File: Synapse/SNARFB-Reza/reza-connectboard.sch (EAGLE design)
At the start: 6 parts

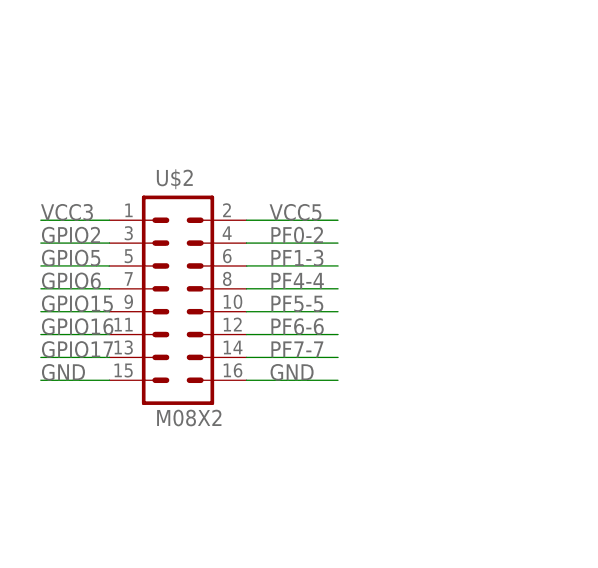
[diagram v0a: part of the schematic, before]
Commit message: comp sync
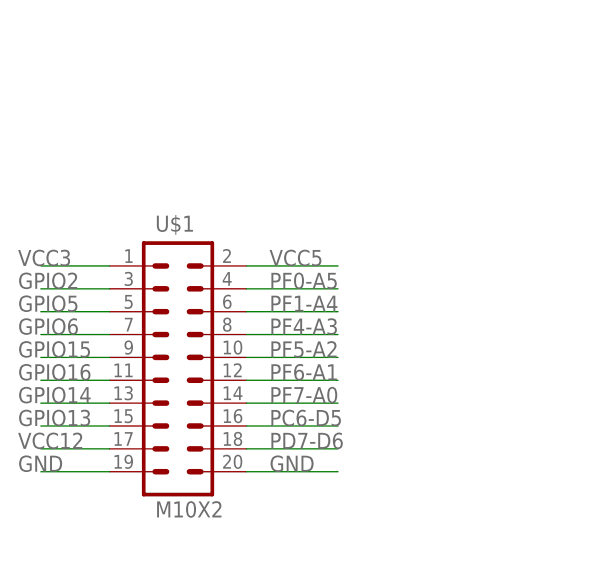
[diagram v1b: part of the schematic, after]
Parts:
- removed U$2: M08X2, SparkFun-Connectors:M08X2
- added U$1: M10X2, SparkFun-Connectors:M10X2
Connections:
- removed net GPIO17: U$2.13
- removed net PF0-2: U$2.4
- removed net PF1-3: U$2.6
- removed net PF4-4: U$2.8
- removed net PF5-5: U$2.10
- removed net PF6-6: U$2.12
- removed net PF7-7: U$2.14
- new net GPIO13: U$1.15
- new net GPIO14: U$1.13
- new net PC6-D5: U$1.16
- new net PD7-D6: U$1.18
- new net PF0-A5: U$1.4
- new net PF1-A4: U$1.6
- new net PF4-A3: U$1.8
- new net PF5-A2: U$1.10
- new net PF6-A1: U$1.12
- new net PF7-A0: U$1.14
- new net VCC12: U$1.17
- net GND: now also U$1.19, U$1.20; no longer U$2.15, U$2.16
- net GPIO15: now also U$1.9; no longer U$2.9
- net GPIO16: now also U$1.11; no longer U$2.11
- net GPIO2: now also U$1.3; no longer U$2.3
- net GPIO5: now also U$1.5; no longer U$2.5
- net GPIO6: now also U$1.7; no longer U$2.7
- net VCC3: now also U$1.1; no longer U$2.1
- net VCC5: now also U$1.2; no longer U$2.2
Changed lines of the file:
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@@
 <class number="0" name="default" width="0.254" drill="0">
+</class>
+<class number="1" name="smallsignal" width="0.1524" drill="0">
+</class>
+<class number="2" name="Power" width="0.508" drill="0">
 </class>
 </classes>
 <parts>
-<part name="U$2" library="SparkFun-Connectors" deviceset="M08X2" device=""/>
 <part name="JP1" library="SparkFun-Connectors" deviceset="M02" device="3.5MM"/>
 <part name="JP2" library="SparkFun-Connectors" deviceset="M02" device="3.5MM"/>
@@
 <part name="JP4" library="SparkFun-Connectors" deviceset="M02" device="3.5MM"/>
 <part name="JP5" library="SparkFun-Connectors" deviceset="M02" device="3.5MM"/>
+<part name="U$1" library="SparkFun-Connectors" deviceset="M10X2" device=""/>
 </parts>
 <sheets>
@@
 </plain>
 <instances>
-<instance part="U$2" gate="G$1" x="35.56" y="30.48"/>
 <instance part="JP1" gate="G$1" x="88.9" y="71.12"/>
 <instance part="JP2" gate="G$1" x="88.9" y="60.96"/>
@@
 <instance part="JP4" gate="G$1" x="88.9" y="22.86"/>
 <instance part="JP5" gate="G$1" x="88.9" y="10.16"/>
+<instance part="U$1" gate="G$1" x="35.56" y="25.4"/>
 </instances>
 <busses>
@@
 <net name="GND" class="0">
 <segment>
-<pinref part="U$2" gate="G$1" pin="15"/>
-<wire x1="27.94" y1="22.86" x2="20.32" y2="22.86" width="0.1524" layer="91"/>
-<label x="20.32" y="22.86" size="1.778" layer="95"/>
+<pinref part="U$1" gate="G$1" pin="19"/>
+<wire x1="27.94" y1="12.7" x2="20.32" y2="12.7" width="0.1524" layer="91"/>
+<label x="17.78" y="12.7" size="1.778" layer="95"/>
 </segment>
 <segment>
-<pinref part="U$2" gate="G$1" pin="16"/>
+<pinref part="U$1" gate="G$1" pin="20"/>
+<wire x1="43.18" y1="12.7" x2="53.34" y2="12.7" width="0.1524" layer="91"/>
+<label x="45.72" y="12.7" size="1.778" layer="95"/>
+</segment>
+</net>
+<net name="GPIO2" class="0">
+<segment>
+<pinref part="U$1" gate="G$1" pin="3"/>
+<wire x1="27.94" y1="33.02" x2="20.32" y2="33.02" width="0.1524" layer="91"/>
+<label x="17.78" y="33.02" size="1.778" layer="95"/>
+</segment>
+</net>
+<net name="GPIO5" class="0">
+<segment>
+<pinref part="U$1" gate="G$1" pin="5"/>
+<wire x1="27.94" y1="30.48" x2="20.32" y2="30.48" width="0.1524" layer="91"/>
+<label x="17.78" y="30.48" size="1.778" layer="95"/>
+</segment>
+</net>
+<net name="GPIO6" class="0">
+<segment>
+<pinref part="U$1" gate="G$1" pin="7"/>
+<wire x1="27.94" y1="27.94" x2="20.32" y2="27.94" width="0.1524" layer="91"/>
+<label x="17.78" y="27.94" size="1.778" layer="95"/>
+</segment>
+</net>
+<net name="GPIO16" class="0">
+<segment>
+<pinref part="U$1" gate="G$1" pin="11"/>
+<wire x1="27.94" y1="22.86" x2="20.32" y2="22.86" width="0.1524" layer="91"/>
+<label x="17.78" y="22.86" size="1.778" layer="95"/>
+</segment>
+</net>
+<net name="GPIO15" class="0">
+<segment>
+<pinref part="U$1" gate="G$1" pin="9"/>
+<wire x1="27.94" y1="25.4" x2="20.32" y2="25.4" width="0.1524" layer="91"/>
+<label x="17.78" y="25.4" size="1.778" layer="95"/>
+</segment>
+</net>
+<net name="VCC3" class="0">
+<segment>
+<pinref part="U$1" gate="G$1" pin="1"/>
+<wire x1="27.94" y1="35.56" x2="20.32" y2="35.56" width="0.1524" layer="91"/>
+<label x="17.78" y="35.56" size="1.778" layer="95"/>
+</segment>
+</net>
+<net name="VCC5" class="0">
+<segment>
+<pinref part="U$1" gate="G$1" pin="2"/>
+<wire x1="43.18" y1="35.56" x2="53.34" y2="35.56" width="0.1524" layer="91"/>
+<label x="45.72" y="35.56" size="1.778" layer="95"/>
+</segment>
+</net>
+<net name="GPIO14" class="1">
+<segment>
+<pinref part="U$1" gate="G$1" pin="13"/>
+<wire x1="27.94" y1="20.32" x2="20.32" y2="20.32" width="0.1524" layer="91"/>
+<label x="17.78" y="20.32" size="1.778" layer="95"/>
+</segment>
+</net>
+<net name="GPIO13" class="1">
+<segment>
+<pinref part="U$1" gate="G$1" pin="15"/>
+<wire x1="27.94" y1="17.78" x2="20.32" y2="17.78" width="0.1524" layer="91"/>
+<label x="17.78" y="17.78" size="1.778" layer="95"/>
+</segment>
+</net>
+<net name="PD7-D6" class="1">
+<segment>
+<pinref part="U$1" gate="G$1" pin="18"/>
+<wire x1="43.18" y1="15.24" x2="53.34" y2="15.24" width="0.1524" layer="91"/>
+<label x="45.72" y="15.24" size="1.778" layer="95"/>
+</segment>
+</net>
+<net name="PC6-D5" class="1">
+<segment>
+<pinref part="U$1" gate="G$1" pin="16"/>
+<wire x1="43.18" y1="17.78" x2="53.34" y2="17.78" width="0.1524" layer="91"/>
+<label x="45.72" y="17.78" size="1.778" layer="95"/>
+</segment>
+</net>
+<net name="PF7-A0" class="1">
+<segment>
+<pinref part="U$1" gate="G$1" pin="14"/>
+<wire x1="43.18" y1="20.32" x2="53.34" y2="20.32" width="0.1524" layer="91"/>
+<label x="45.72" y="20.32" size="1.778" layer="95"/>
+</segment>
+</net>
+<net name="PF4-A3" class="1">
+<segment>
+<pinref part="U$1" gate="G$1" pin="8"/>
+<wire x1="43.18" y1="27.94" x2="53.34" y2="27.94" width="0.1524" layer="91"/>
+<label x="45.72" y="27.94" size="1.778" layer="95"/>
+</segment>
+</net>
+<net name="PF1-A4" class="1">
+<segment>
+<pinref part="U$1" gate="G$1" pin="6"/>
+<wire x1="43.18" y1="30.48" x2="53.34" y2="30.48" width="0.1524" layer="91"/>
+<label x="45.72" y="30.48" size="1.778" layer="95"/>
+</segment>
+</net>
+<net name="PF0-A5" class="1">
+<segment>
+<pinref part="U$1" gate="G$1" pin="4"/>
+<wire x1="43.18" y1="33.02" x2="53.34" y2="33.02" width="0.1524" layer="91"/>
+<label x="45.72" y="33.02" size="1.778" layer="95"/>
+</segment>
+</net>
+<net name="PF6-A1" class="1">
+<segment>
+<pinref part="U$1" gate="G$1" pin="12"/>
 <wire x1="43.18" y1="22.86" x2="53.34" y2="22.86" width="0.1524" layer="91"/>
 <label x="45.72" y="22.86" size="1.778" layer="95"/>
 </segment>
 </net>
-<net name="GPIO2" class="0">
+<net name="PF5-A2" class="1">
 <segment>
-<pinref part="U$2" gate="G$1" pin="3"/>
-<wire x1="27.94" y1="38.1" x2="20.32" y2="38.1" width="0.1524" layer="91"/>
-<label x="20.32" y="38.1" size="1.778" layer="95"/>
-</segment>
-</net>
-<net name="GPIO5" class="0">
-<segment>
-<pinref part="U$2" gate="G$1" pin="5"/>
-<wire x1="27.94" y1="35.56" x2="20.32" y2="35.56" width="0.1524" layer="91"/>
-<label x="20.32" y="35.56" size="1.778" layer="95"/>
-</segment>
-</net>
-<net name="GPIO6" class="0">
-<segment>
-<pinref part="U$2" gate="G$1" pin="7"/>
-<wire x1="27.94" y1="33.02" x2="20.32" y2="33.02" width="0.1524" layer="91"/>
-<label x="20.32" y="33.02" size="1.778" layer="95"/>
-</segment>
-</net>
-<net name="GPIO16" class="0">
-<segment>
-<pinref part="U$2" gate="G$1" pin="11"/>
-<wire x1="27.94" y1="27.94" x2="20.32" y2="27.94" width="0.1524" layer="91"/>
-<label x="20.32" y="27.94" size="1.778" layer="95"/>
-</segment>
-</net>
-<net name="GPIO15" class="0">
-<segment>
-<pinref part="U$2" gate="G$1" pin="9"/>
-<wire x1="27.94" y1="30.48" x2="20.32" y2="30.48" width="0.1524" layer="91"/>
-<label x="20.32" y="30.48" size="1.778" layer="95"/>
-</segment>
-</net>
-<net name="VCC3" class="0">
-<segment>
-<pinref part="U$2" gate="G$1" pin="1"/>
-<wire x1="27.94" y1="40.64" x2="20.32" y2="40.64" width="0.1524" layer="91"/>
-<label x="20.32" y="40.64" size="1.778" layer="95"/>
-</segment>
-</net>
-<net name="PF7-7" class="0">
-<segment>
-<pinref part="U$2" gate="G$1" pin="14"/>
+<pinref part="U$1" gate="G$1" pin="10"/>
 <wire x1="43.18" y1="25.4" x2="53.34" y2="25.4" width="0.1524" layer="91"/>
 <label x="45.72" y="25.4" size="1.778" layer="95"/>
 </segment>
 </net>
-<net name="PF4-4" class="0">
+<net name="VCC12" class="2">
 <segment>
-<pinref part="U$2" gate="G$1" pin="8"/>
-<wire x1="43.18" y1="33.02" x2="53.34" y2="33.02" width="0.1524" layer="91"/>
-<label x="45.72" y="33.02" size="1.778" layer="95"/>
+<pinref part="U$1" gate="G$1" pin="17"/>
+<wire x1="27.94" y1="15.24" x2="20.32" y2="15.24" width="0.1524" layer="91"/>
+<label x="17.78" y="15.24" size="1.778" layer="95"/>
 </segment>
 </net>
-<net name="PF1-3" class="0">
-<segment>
-<pinref part="U$2" gate="G$1" pin="6"/>
-<wire x1="43.18" y1="35.56" x2="53.34" y2="35.56" width="0.1524" layer="91"/>
-<label x="45.72" y="35.56" size="1.778" layer="95"/>
-</segment>
-</net>
-<net name="PF0-2" class="0">
-<segment>
-<pinref part="U$2" gate="G$1" pin="4"/>
-<wire x1="43.18" y1="38.1" x2="53.34" y2="38.1" width="0.1524" layer="91"/>
-<label x="45.72" y="38.1" size="1.778" layer="95"/>
-</segment>
-</net>
-<net name="PF6-6" class="0">
-<segment>
-<pinref part="U$2" gate="G$1" pin="12"/>
-<wire x1="43.18" y1="27.94" x2="53.34" y2="27.94" width="0.1524" layer="91"/>
-<label x="45.72" y="27.94" size="1.778" layer="95"/>
-</segment>
-</net>
-<net name="PF5-5" class="0">
-<segment>
-<pinref part="U$2" gate="G$1" pin="10"/>
-<wire x1="43.18" y1="30.48" x2="53.34" y2="30.48" width="0.1524" layer="91"/>
-<label x="45.72" y="30.48" size="1.778" layer="95"/>
-</segment>
-</net>
-<net name="VCC5" class="0">
-<segment>
-<pinref part="U$2" gate="G$1" pin="2"/>
-<wire x1="43.18" y1="40.64" x2="53.34" y2="40.64" width="0.1524" layer="91"/>
-<label x="45.72" y="40.64" size="1.778" layer="95"/>
-</segment>
-</net>
-<net name="GPIO17" class="0">
-<segment>
-<pinref part="U$2" gate="G$1" pin="13"/>
-<wire x1="27.94" y1="25.4" x2="20.32" y2="25.4" width="0.1524" layer="91"/>
-<label x="20.32" y="25.4" size="1.778" layer="95"/>
-</segment>
-</net>

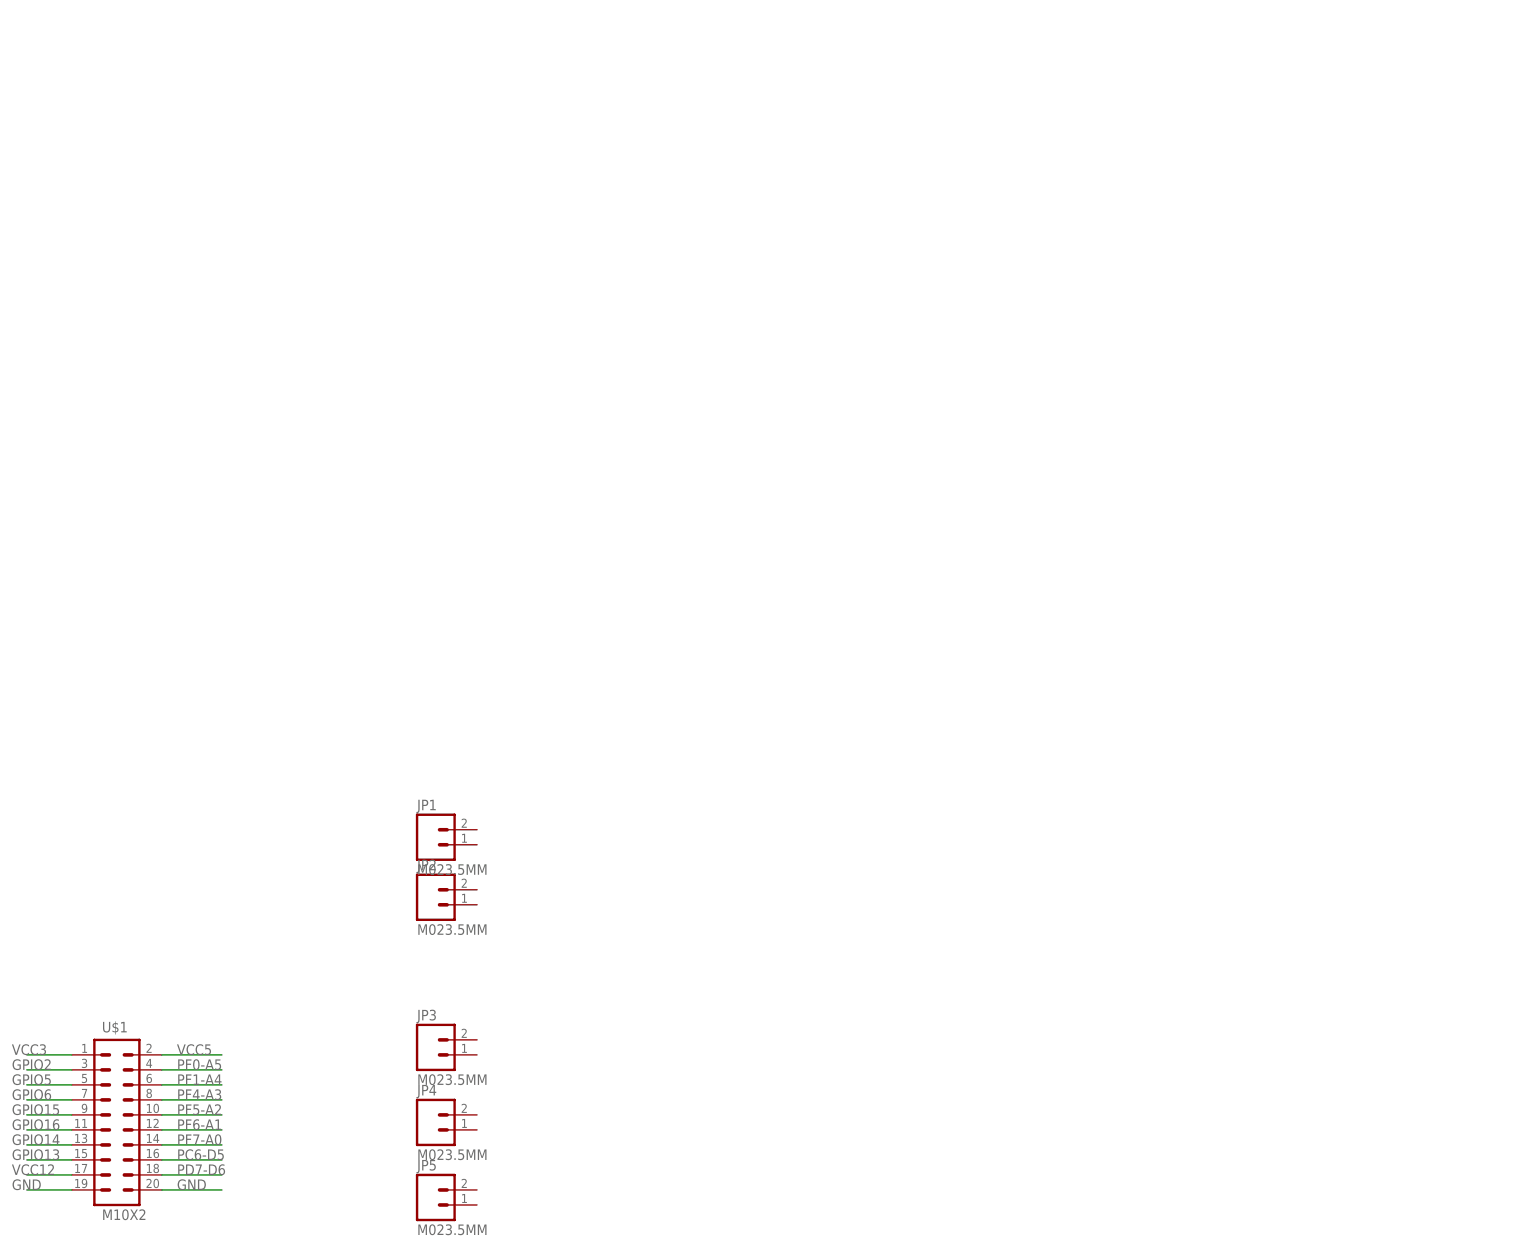
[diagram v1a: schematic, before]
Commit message: sync
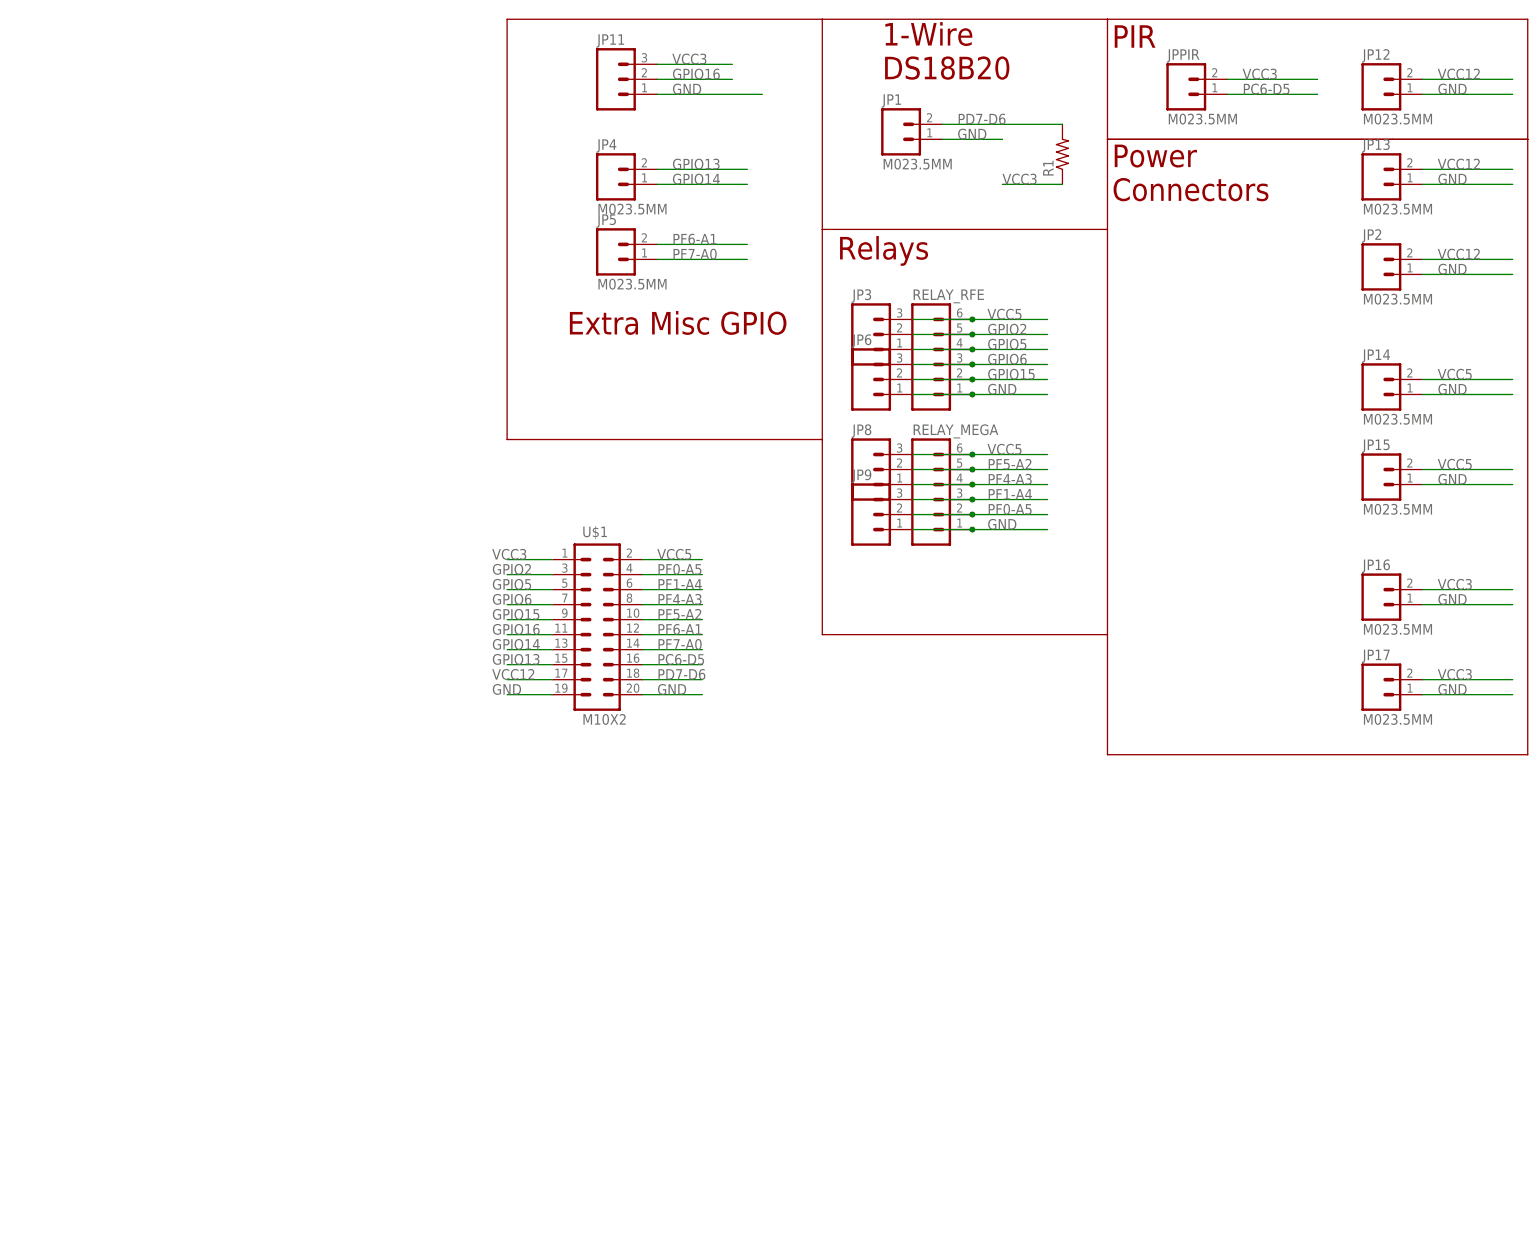
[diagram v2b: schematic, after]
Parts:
- added JP11, JP6, JP8, JP9: (no value), SparkFun-Connectors:M03SCREW
- added JP12, JP13, JP14, JP15, JP16, JP17, JPPIR: M023.5MM, SparkFun-Connectors:M023.5MM
- added R1: (no value), adafruit:R-US_FLIPFLOP
- added RELAY_MEGA, RELAY_RFE: (no value), SparkFun-Connectors:M06SIP
- JP3: value M023.5MM -> (none); device SparkFun-Connectors:M023.5MM -> SparkFun-Connectors:M03SCREW
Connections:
- net GND: now also JP1.1, JP11.1, JP12.1, JP13.1, JP14.1, JP15.1, JP16.1, JP17.1, JP2.1, JP6.1, JP9.1, RELAY_MEGA.1, RELAY_RFE.1
- net GPIO13: now also JP4.2
- net GPIO14: now also JP4.1
- net GPIO15: now also JP6.2, RELAY_RFE.2
- net GPIO16: now also JP11.2
- net GPIO2: now also JP3.2, RELAY_RFE.5
- net GPIO5: now also JP3.1, RELAY_RFE.4
- net GPIO6: now also JP6.3, RELAY_RFE.3
- net PC6-D5: now also JPPIR.1
- net PD7-D6: now also JP1.2, R1.2
- net PF0-A5: now also JP9.2, RELAY_MEGA.2
- net PF1-A4: now also JP9.3, RELAY_MEGA.3
- net PF4-A3: now also JP8.1, RELAY_MEGA.4
- net PF5-A2: now also JP8.2, RELAY_MEGA.5
- net PF6-A1: now also JP5.2
- net PF7-A0: now also JP5.1
- net VCC12: now also JP12.2, JP13.2, JP2.2
- net VCC3: now also JP11.3, JP16.2, JP17.2, JPPIR.2, R1.1
- net VCC5: now also JP14.2, JP15.2, JP3.3, JP8.3, RELAY_MEGA.6, RELAY_RFE.6
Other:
- note added: "1-Wire DS18B20"
- note added: "Extra Misc GPIO"
- note added: "PIR"
- note added: "Power Connectors"
- note added: "Relays"
- moved on the sheet: JP1, JP2, JP4, JP5, U$1
